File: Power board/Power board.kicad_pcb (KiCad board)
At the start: 2 copper layers, 66 x 100 mm, 31 parts, among them J1 High1, J10 2x2_pin_bat+, J11 2x2_pin_bat-, J2 Low1, J3 High2, J4 Low2, J5 Bat+, J6 Bat-, J7 Phase, J8 2x2_pin_support1, J9 2x2_pin_support2, Q1 IPB017N10N5, Q2 IPB017N10N5, Q3 IPB017N10N5, Q4 IPB017N10N5

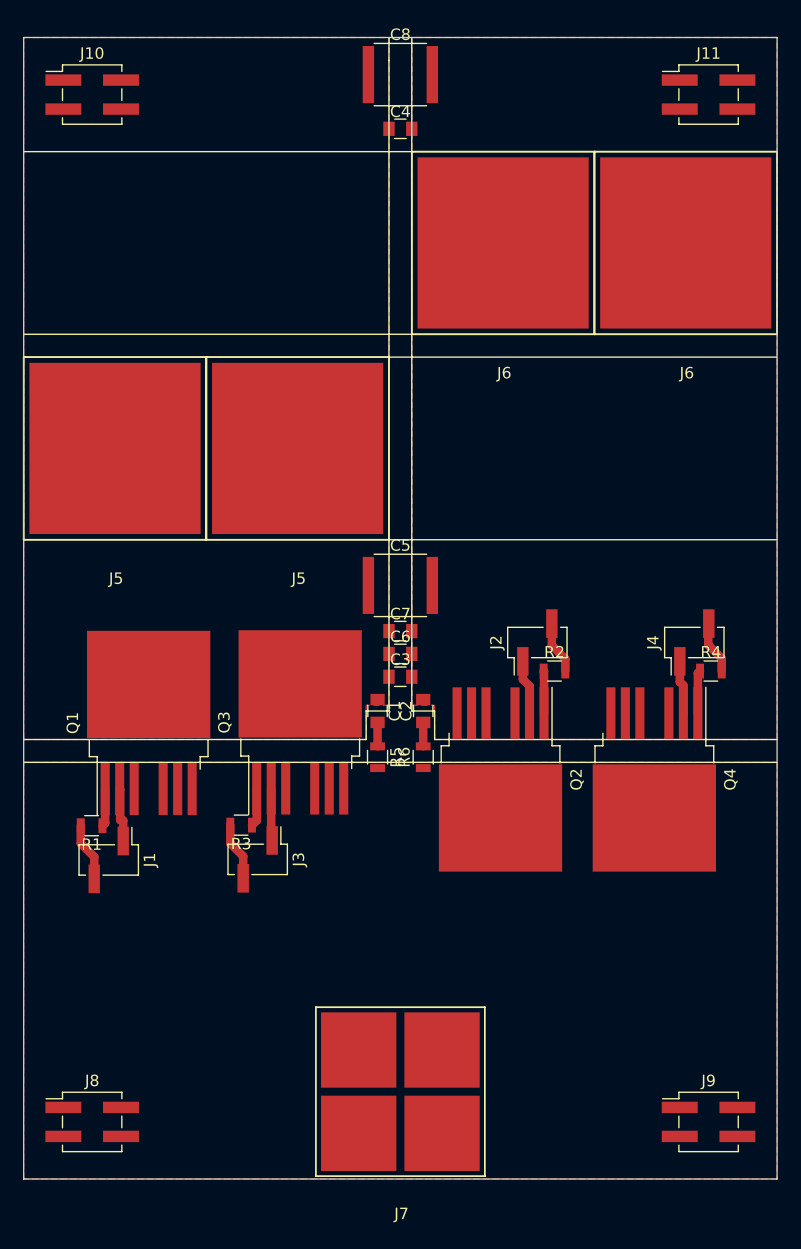
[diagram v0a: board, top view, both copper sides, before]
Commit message: Updated
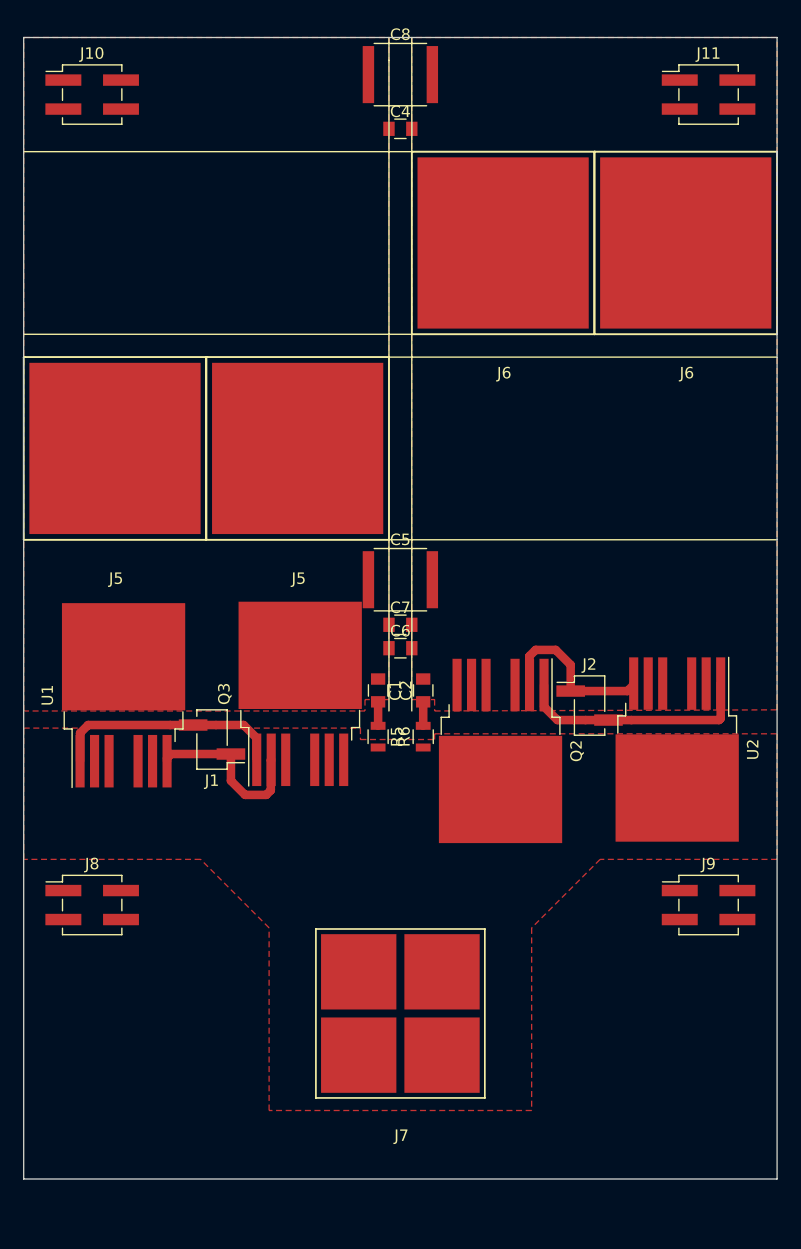
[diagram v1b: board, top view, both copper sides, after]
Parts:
- removed C3: 1u, Capacitors_SMD:C_0805
- removed J3: High2, Pin_Headers:Pin_Header_Straight_1x02_Pitch2.54mm_SMD_Pin1Left
- removed J4: Low2, Pin_Headers:Pin_Header_Straight_1x02_Pitch2.54mm_SMD_Pin1Left
- removed Q1, Q4: IPB017N10N5, TO_SOT_Packages_SMD:TO-263-7_TabPin4
- removed R1, R2, R3, R4: 4.7, Resistors_SMD:R_0805
- added U1: IPB017N10N5-1, TO_SOT_Packages_SMD:TO-263-7_TabPin4, F.Cu at (34.8, 134.6)
- added U2: IPB017N10N5-1, TO_SOT_Packages_SMD:TO-263-7_TabPin4, F.Cu at (83.2, 139.4)
- moved J8 19.0 mm to (32.0, 153.0)
- moved J9 19.0 mm to (86.0, 153.0)
- moved J1 13.9 mm to (42.5, 138.5), turned to 180 degrees
- moved J2 7.17 mm to (75.6, 135.5), turned to 0 degrees
- moved J7 6.85 mm to (59.0, 162.5)
- moved Q2 2.50 mm to (67.8, 139.5)
- moved Q3 2.50 mm to (50.2, 134.5)
- moved C1 1.80 mm to (57.0, 134.2)
- moved R5 1.80 mm to (57.0, 138.2)
- moved C2 1.80 mm to (61.0, 134.2)
- moved R6 1.80 mm to (61.0, 138.2)
- moved C7 0.55 mm to (59.0, 128.4)
- moved C5 0.50 mm to (59.0, 124.5)
- moved C6 0.50 mm to (59.0, 130.5)
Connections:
- Q2 pad 1: Net-(Q2-Pad1) -> Net-(J2-Pad2)
- Q3 pad 1: Net-(Q3-Pad1) -> Net-(J1-Pad2)
- Q3 pad 2: Net-(J3-Pad1) -> Net-(J1-Pad1)
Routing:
- net Net-(J2-Pad2): track 4.64 -> 21.0 mm
- net Net-(J1-Pad2): track 5.14 -> 20.6 mm
- net Net-(J1-Pad1): track 4.83 -> 15.2 mm
- net Net-(J2-Pad1): track 4.81 -> 15.1 mm
- net Net-(J3-Pad2): track 5.12 -> 0.00 mm
- net Net-(J4-Pad1): track 4.70 -> 0.00 mm
- net Net-(J4-Pad2): track 4.66 -> 0.00 mm
- net Net-(J3-Pad1): track 4.61 -> 0.00 mm
- net Net-(Q4-Pad1): track 3.80 -> 0.00 mm
- net Net-(Q2-Pad1): track 3.74 -> 0.00 mm
- net Net-(Q3-Pad1): track 3.40 -> 0.00 mm
- net Net-(Q1-Pad1): track 3.32 -> 0.00 mm
